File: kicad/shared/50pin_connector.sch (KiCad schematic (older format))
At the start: 1 part, among them P5 CONN_02X25

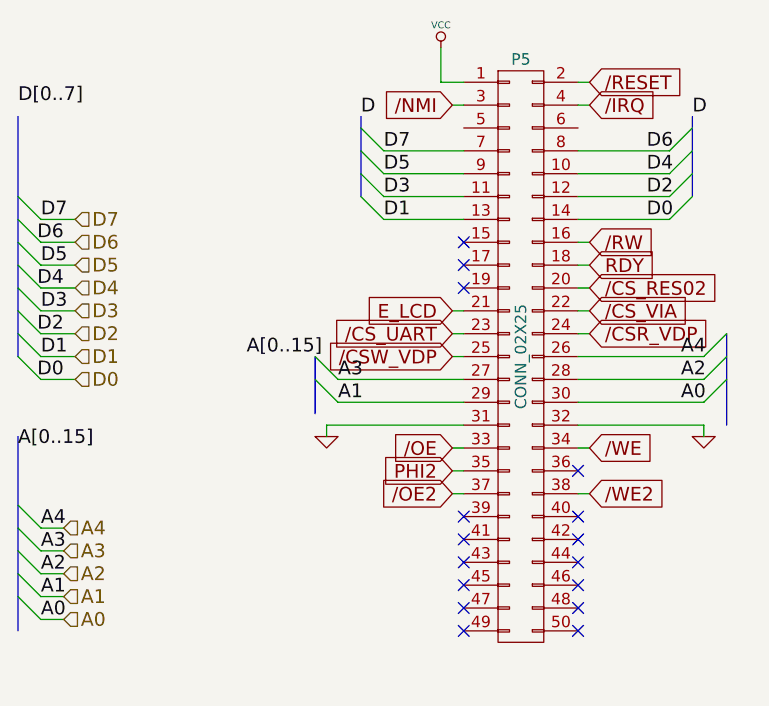
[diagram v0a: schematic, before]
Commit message: connector
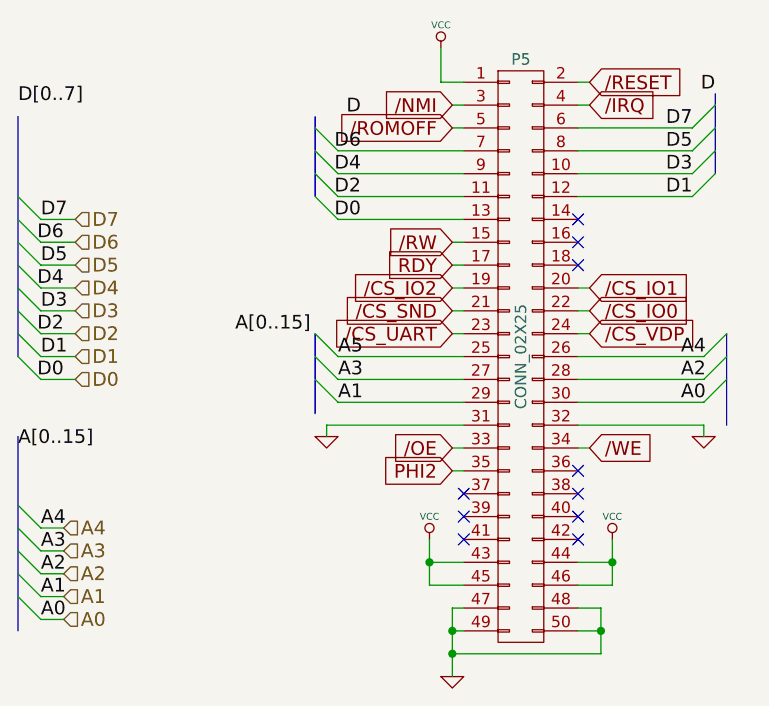
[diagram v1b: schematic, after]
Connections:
- net /RW: now also P5.15 (P15); no longer P5.16 (P16)
- net D0: now also P5.13 (P13); no longer P5.14 (P14)
- net D1: now also P5.12 (P12); no longer P5.13 (P13)
- net D2: now also P5.11 (P11); no longer P5.12 (P12)
- net D3: now also P5.10 (P10); no longer P5.11 (P11)
- net D4: now also P5.9 (P9); no longer P5.10 (P10)
- net D5: now also P5.8 (P8); no longer P5.9 (P9)
- net D6: now also P5.7 (P7); no longer P5.8 (P8)
- net D7: now also P5.6 (P6); no longer P5.7 (P7)
- net GND: now also P5.47 (P47), P5.48 (P48), P5.49 (P49), P5.50 (P50)
- net RDY: now also P5.17 (P17); no longer P5.18 (P18)
- net VCC: now also P5.43 (P43), P5.44 (P44), P5.45 (P45), P5.46 (P46)
- net /CS_IO2: now reaches P5.19 (P19)
- net /ROMOFF: now reaches P5.5 (P5)
- net /CSR_VDP renamed /CS_VDP
- net /CSW_VDP renamed A5
- net /CS_RES02 renamed /CS_IO1
- net /CS_VIA renamed /CS_IO0
- net /OE2: no longer names the net of P5.37 (P37)
- net /WE2: no longer names the net of P5.38 (P38)
- net E_LCD renamed /CS_SND
- no-connect marks 16 -> 10
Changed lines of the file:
@@
 LIBS:contrib
 LIBS:valves
-LIBS:65xxx
-LIBS:gal
-LIBS:UART
-LIBS:osc
-LIBS:steckschwein-cache
 EELAYER 24 0
 EELAYER END
 $Descr A4 11693 8268
 encoding utf-8
-Sheet 2 2
+Sheet 1 1
 Title ""
 Date ""
@@
 /NMI
 Wire Bus Line
-	4850 2700 4850 3050
-Entry Wire Line
-	4850 2750 4950 2850
-Entry Wire Line
-	4850 2850 4950 2950
-Entry Wire Line
-	4850 2950 4950 3050
-Entry Wire Line
-	4850 3050 4950 3150
-Wire Wire Line
-	4950 2850 5300 2850
-Wire Wire Line
-	4950 2950 5300 2950
-Wire Wire Line
-	4950 3050 5300 3050
-Wire Wire Line
-	4950 3150 5300 3150
-Text Label 4950 2850 0    60   ~ 0
+	6400 2600 6400 2950
+Entry Wire Line
+	6400 2650 6300 2750
+Entry Wire Line
+	6400 2750 6300 2850
+Entry Wire Line
+	6400 2850 6300 2950
+Entry Wire Line
+	6400 2950 6300 3050
+Text Label 6300 2750 2    60   ~ 0
 D7
-Text Label 4950 2950 0    60   ~ 0
+Text Label 6300 2850 2    60   ~ 0
 D5
-Text Label 4950 3050 0    60   ~ 0
+Text Label 6300 2950 2    60   ~ 0
 D3
-Text Label 4950 3150 0    60   ~ 0
+Text Label 6300 3050 2    60   ~ 0
 D1
 Wire Bus Line
-	6300 2700 6300 3050
-Entry Wire Line
-	6200 2850 6300 2750
-Entry Wire Line
-	6200 2950 6300 2850
-Entry Wire Line
-	6200 3050 6300 2950
-Entry Wire Line
-	6200 3150 6300 3050
-Wire Wire Line
-	5800 2850 6200 2850
-Wire Wire Line
-	5800 2950 6200 2950
-Wire Wire Line
-	5800 3050 6200 3050
-Wire Wire Line
-	5800 3150 6200 3150
-Wire Wire Line
-	5800 3250 5850 3250
-Text GLabel 5850 3250 2    60   Input ~ 0
+	4650 2700 4650 3050
+Entry Wire Line
+	4750 2850 4650 2750
+Entry Wire Line
+	4750 2950 4650 2850
+Entry Wire Line
+	4750 3050 4650 2950
+Entry Wire Line
+	4750 3150 4650 3050
+Text GLabel 5250 3250 0    60   Input ~ 0
 /RW
-Text GLabel 5850 3350 2    60   Input ~ 0
+Text GLabel 5250 3350 0    60   Input ~ 0
 RDY
-Wire Wire Line
-	5800 3350 5850 3350
 Wire Wire Line
 	5300 3550 5250 3550
 Text GLabel 5250 3550 0    60   Input ~ 0
-E_LCD
+/CS_SND
 Wire Wire Line
 	5800 3550 5850 3550
 Text GLabel 5850 3550 2    60   Input ~ 0
-/CS_VIA
+/CS_IO0
 Text GLabel 5250 3650 0    60   Input ~ 0
 /CS_UART
@@
 	5300 3650 5250 3650
 Text GLabel 5850 3650 2    60   Input ~ 0
-/CSR_VDP
-Text GLabel 5250 3750 0    60   Input ~ 0
-/CSW_VDP
-Wire Wire Line
-	5250 3750 5300 3750
+/CS_VDP
+Wire Wire Line
+	4750 3750 5300 3750
 Wire Wire Line
 	5800 3650 5850 3650
@@
 	5800 3950 6350 3950
 Wire Bus Line
-	4650 3750 4650 4000
+	4650 3650 4650 4000
 Entry Wire Line
 	4650 3750 4750 3850
@@
 Text GLabel 5850 4150 2    60   Input ~ 0
 /WE
-Text Label 6100 2850 0    60   ~ 0
+Text Label 4850 2850 2    60   ~ 0
 D6
-Text Label 6100 2950 0    60   ~ 0
+Text Label 4850 2950 2    60   ~ 0
 D4
-Text Label 6100 3050 0    60   ~ 0
+Text Label 4850 3050 2    60   ~ 0
 D2
-Text Label 6100 3150 0    60   ~ 0
+Text Label 4850 3150 2    60   ~ 0
 D0
 Text Label 6250 3950 0    60   ~ 0
@@
 Text Label 4750 3850 0    60   ~ 0
 A3
-Text Label 6300 2700 0    60   ~ 0
+Text Label 4850 2700 2    60   ~ 0
 D
-Text Label 4850 2700 0    60   ~ 0
+Text Label 6400 2600 2    60   ~ 0
 D
-Text Label 4350 3750 0    60   ~ 0
+Text Label 4300 3650 0    60   ~ 0
 A[0..15]
-Text GLabel 5250 4350 0    60   Input ~ 0
-/OE2
-Text GLabel 5850 4350 2    60   Input ~ 0
-/WE2
-Wire Wire Line
-	5850 4350 5800 4350
-Wire Wire Line
-	5250 4350 5300 4350
-NoConn ~ 5300 3250
-NoConn ~ 5300 3350
-NoConn ~ 5300 3450
 NoConn ~ 5800 4250
 NoConn ~ 5300 4450
 NoConn ~ 5300 4550
-NoConn ~ 5300 4650
-NoConn ~ 5300 4750
-NoConn ~ 5300 4850
-NoConn ~ 5300 4950
 NoConn ~ 5800 4450
 NoConn ~ 5800 4550
-NoConn ~ 5800 4650
-NoConn ~ 5800 4750
-NoConn ~ 5800 4850
-NoConn ~ 5800 4950
 Wire Wire Line
 	5800 3450 5850 3450
 Text GLabel 5850 3450 2    60   Input ~ 0
-/CS_RES02
+/CS_IO1
 Text HLabel 3550 4900 2    60   Input ~ 0
 A0
@@
 Text Label 3450 4500 0    60   ~ 0
 A4
+Text GLabel 5250 3450 0    60   Input ~ 0
+/CS_IO2
+Wire Wire Line
+	5250 3450 5300 3450
+Wire Wire Line
+	5250 3350 5300 3350
+NoConn ~ 5800 3350
+Wire Wire Line
+	5300 2850 4750 2850
+Wire Wire Line
+	5300 2950 4750 2950
+Wire Wire Line
+	5300 3050 4750 3050
+Wire Wire Line
+	5300 3150 4750 3150
+Wire Wire Line
+	5800 2750 6300 2750
+Wire Wire Line
+	6300 2850 5800 2850
+Wire Wire Line
+	6300 2950 5800 2950
+Wire Wire Line
+	6300 3050 5800 3050
+Text GLabel 5250 2750 0    60   Input ~ 0
+/ROMOFF
+Wire Wire Line
+	5250 2750 5300 2750
+NoConn ~ 5800 3150
+Wire Wire Line
+	5250 3250 5300 3250
+NoConn ~ 5800 3250
+Entry Wire Line
+	4650 3650 4750 3750
+Text Label 4750 3750 0    60   ~ 0
+A5
+NoConn ~ 5800 4350
+NoConn ~ 5300 4350
+$Comp
+L GND #PWR?
+U 1 1 5436D639
+P 5250 5150
+F 0 "#PWR?" H 5250 5150 30  0001 C CNN
+F 1 "GND" H 5250 5080 30  0001 C CNN
+F 2 "" H 5250 5150 60  0000 C CNN
+F 3 "" H 5250 5150 60  0000 C CNN
+	1    5250 5150
+	1    0    0    -1
+$EndComp
+Wire Wire Line
+	5300 4850 5250 4850
+Wire Wire Line
+	5250 4850 5250 5150
+Wire Wire Line
+	5300 4950 5250 4950
+Connection ~ 5250 4950
+$Comp
+L VCC #PWR?
+U 1 1 5436D6BC
+P 5950 4550
+F 0 "#PWR?" H 5950 4650 30  0001 C CNN
+F 1 "VCC" H 5950 4650 30  0000 C CNN
+F 2 "" H 5950 4550 60  0000 C CNN
+F 3 "" H 5950 4550 60  0000 C CNN
+	1    5950 4550
+	1    0    0    -1
+$EndComp
+Wire Wire Line
+	5800 4850 5900 4850
+Wire Wire Line
+	5900 4850 5900 5050
+Wire Wire Line
+	5900 5050 5250 5050
+Connection ~ 5250 5050
+Wire Wire Line
+	5800 4950 5900 4950
+Connection ~ 5900 4950
+Wire Wire Line
+	5800 4650 5950 4650
+Wire Wire Line
+	5950 4550 5950 4750
+Wire Wire Line
+	5950 4750 5800 4750
+Connection ~ 5950 4650
+$Comp
+L VCC #PWR?
+U 1 1 5436D806
+P 5150 4550
+F 0 "#PWR?" H 5150 4650 30  0001 C CNN
+F 1 "VCC" H 5150 4650 30  0000 C CNN
+F 2 "" H 5150 4550 60  0000 C CNN
+F 3 "" H 5150 4550 60  0000 C CNN
+	1    5150 4550
+	1    0    0    -1
+$EndComp
+Wire Wire Line
+	5150 4550 5150 4750
+Wire Wire Line
+	5150 4750 5300 4750
+Wire Wire Line
+	5300 4650 5150 4650
+Connection ~ 5150 4650
 $EndSCHEMATC
